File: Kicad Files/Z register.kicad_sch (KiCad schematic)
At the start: 24 parts, among them SW3 SW_DIP_x02, U15 74LS00, U16 LM555xN, U17 74LS273, U18 74LS112, U19 74LS112, U20 28C256, U21 74LS139, U22 HDSP-7403, U23 HDSP-7403, U24 HDSP-7403, U25 HDSP-7403

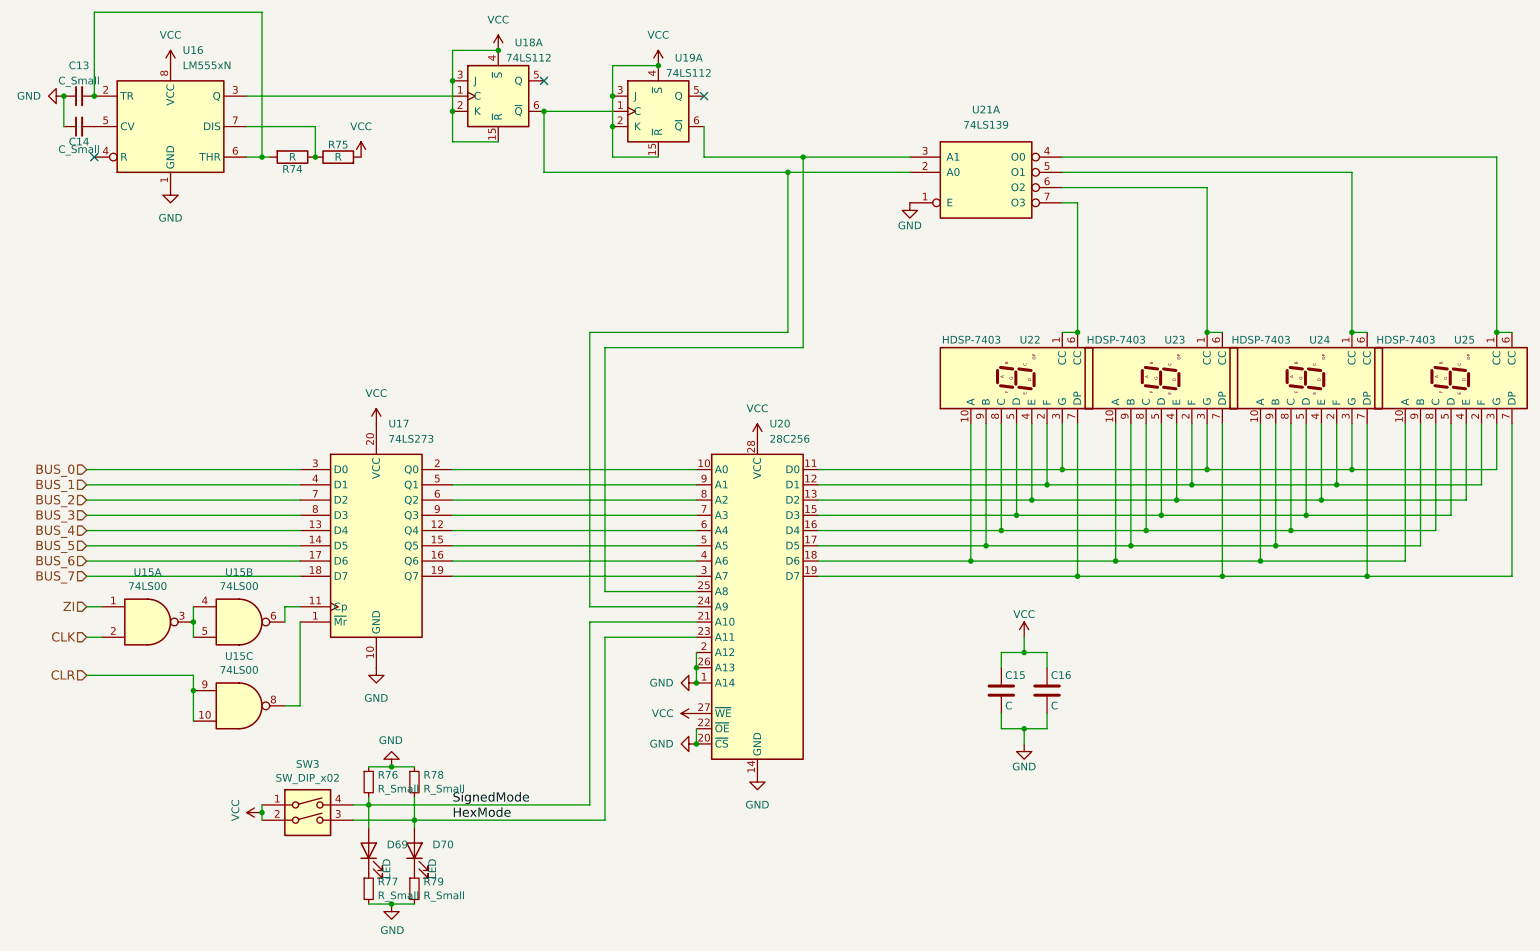
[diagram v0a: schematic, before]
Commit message: im sooo stupiiid
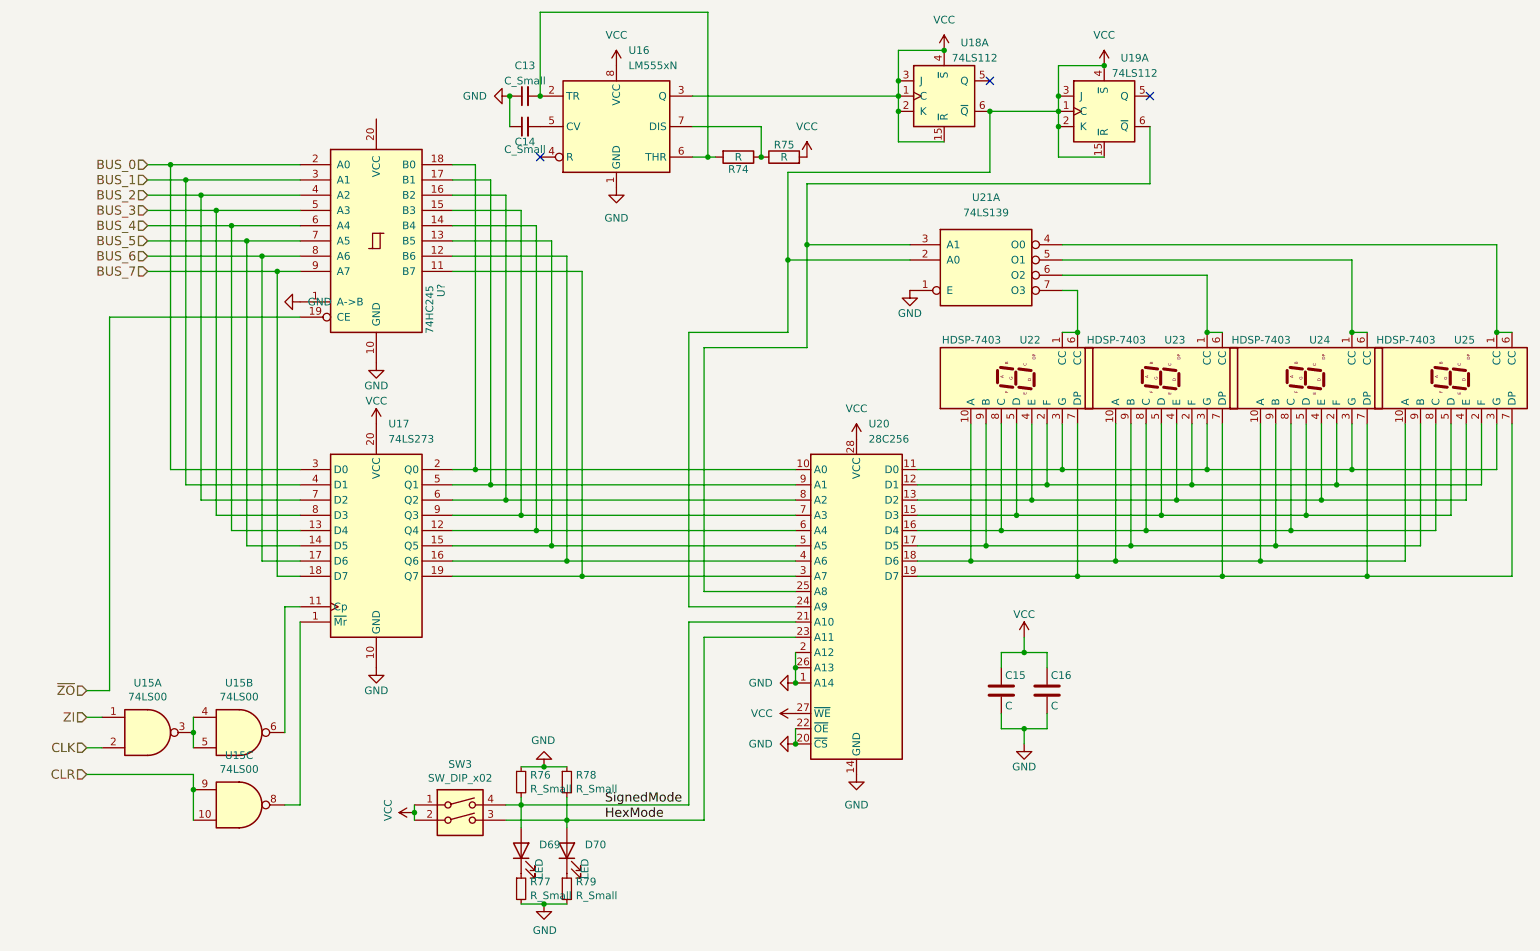
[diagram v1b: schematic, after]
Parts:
- added U?: 74HC245, symbol 74xx:74HC245
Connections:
- net BUS_0: now also U?.2 (A0)
- net BUS_1: now also U?.3 (A1)
- net BUS_2: now also U?.4 (A2)
- net BUS_3: now also U?.5 (A3)
- net BUS_4: now also U?.6 (A4)
- net BUS_5: now also U?.7 (A5)
- net BUS_6: now also U?.8 (A6)
- net BUS_7: now also U?.9 (A7)
- net GND: now also U?.1 (A->B), U?.10 (GND)
- net VCC: now also U16.3 (Q), U18.1 (C), U18.6 (~{Q}), U19.1 (C), U20.24 (A9), U21.2 (A0)
- net at U17.12 (Q4), U20.6 (A4): now also U?.14 (B4)
- net at U17.15 (Q5), U20.5 (A5): now also U?.13 (B5)
- net at U17.16 (Q6), U20.4 (A6): now also U?.12 (B6)
- net at U17.19 (Q7), U20.3 (A7): now also U?.11 (B7)
- net at U17.2 (Q0), U20.10 (A0): now also U?.18 (B0)
- net at U17.5 (Q1), U20.9 (A1): now also U?.17 (B1)
- net at U17.6 (Q2), U20.8 (A2): now also U?.16 (B2)
- net at U17.9 (Q3), U20.7 (A3): now also U?.15 (B3)
- new net ~{ZO}: U?.19 (CE)
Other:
- moved on the sheet: C13, C14, D69, D70, R74, R75, R76, R77, R78, R79, SW3, U15A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
